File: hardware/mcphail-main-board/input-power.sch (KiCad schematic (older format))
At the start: 34 parts, among them J8 INPUT 6V-9V, J9 JST PH, U10 BUCK-BOOST 5V TPS63060, U11 MCP1703, U9 MCP73871

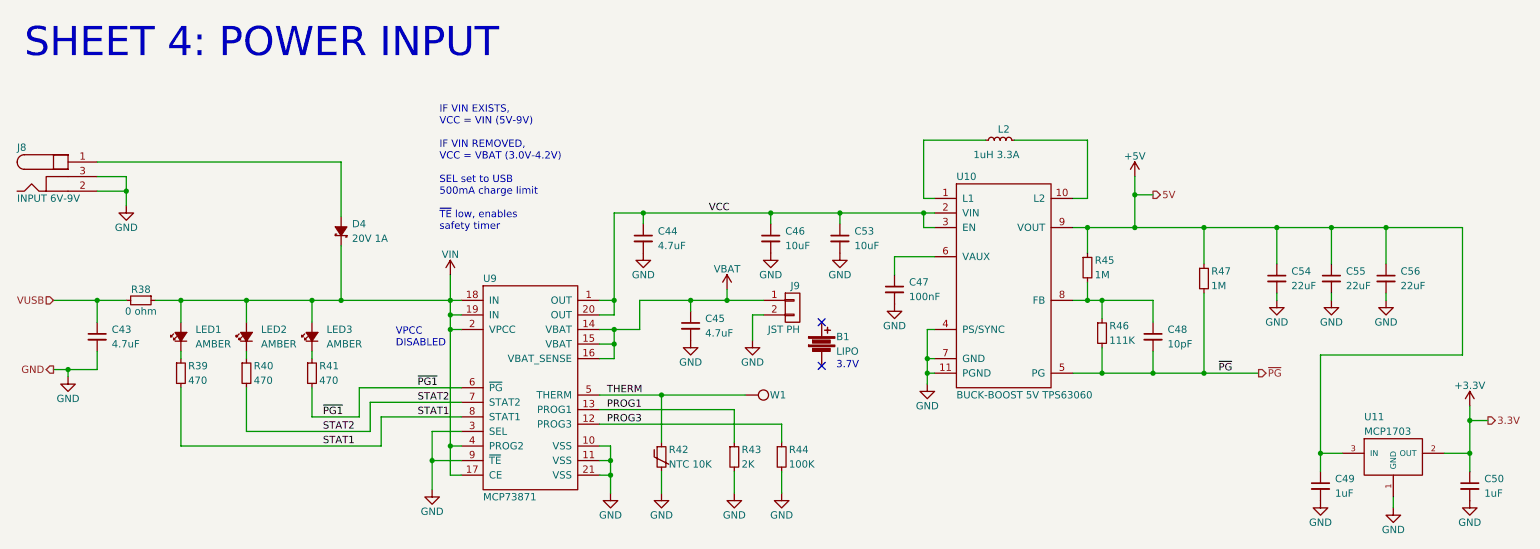
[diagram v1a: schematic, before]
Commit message: Commit.
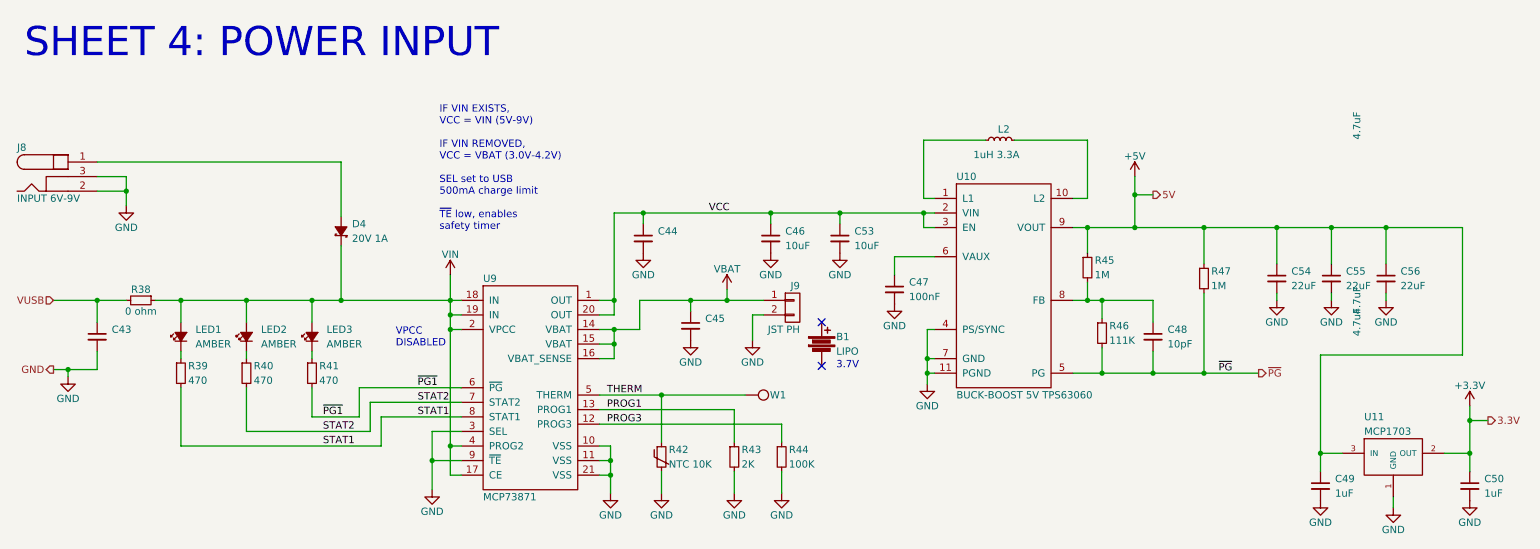
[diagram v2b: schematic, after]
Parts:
- C43, C44, C45: MF_Name Taiyo Yuden -> Samsung; MF_PN UMK316AB7475KL-T -> CL31B475KBHNNNE; S1_PN 587-2994-1-ND -> 1276-2789-1-ND
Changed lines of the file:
@@
 EESchema Schematic File Version 2
 LIBS:wickerlib
-LIBS:mcphail-main-board-cache
 EELAYER 25 0
 EELAYER END
@@
 P 4975 2325
 F 0 "C44" H 5075 2375 50  0000 L CNN
-F 1 "4.7uF" H 5075 2275 50  0000 L CNN
-F 2 "Wickerlib:RLC-1206-SMD" H 5600 1925 50  0001 C CIN
-F 3 "http://ds.yuden.co.jp/TYCOMPAS/ut/detail.do?productNo=UMK316AB7475KL-T&fileName=UMK316AB7475KL-T_SS&mode=specSheetDownload" H 5325 2100 50  0001 C CNN
-F 4 "CAP CER 4.7UF 50V X7R 1206" H 5650 2000 50  0001 C CIN "Description"
-F 5 "Taiyo Yuden" H 5175 1825 50  0001 C CIN "MF_Name"
-F 6 "UMK316AB7475KL-T" H 5850 1825 50  0001 C CIN "MF_PN"
-F 7 "Digikey" H 5075 1725 50  0001 C CIN "S1_Name"
-F 8 "587-2994-1-ND" H 5775 1725 50  0001 C CIN "S1_PN"
+F 1 "4.7uF" V 9875 3100 50  0000 C CNN
+F 2 "Wickerlib:RLC-1206-SMD" H 10375 2700 50  0001 C CIN
+F 3 "http://www.samsungsem.com/kr/support/product-search/mlcc/CL31B475KBHNNNE.jsp" H 10100 2875 50  0001 C CNN
+F 4 "CAP CER 4.7UF 50V X7R 1206" H 10425 2775 50  0001 C CIN "Description"
+F 5 "Samsung" H 9950 2600 50  0001 C CIN "MF_Name"
+F 6 "CL31B475KBHNNNE" H 10625 2600 50  0001 C CIN "MF_PN"
+F 7 "Digikey" H 9850 2500 50  0001 C CIN "S1_Name"
+F 8 "1276-2789-1-ND" H 10550 2500 50  0001 C CIN "S1_PN"
 	1    4975 2325
 	1    0    0    -1
@@
 P 5300 2925
 F 0 "C45" H 5400 2975 50  0000 L CNN
-F 1 "4.7uF" H 5400 2875 50  0000 L CNN
-F 2 "Wickerlib:RLC-1206-SMD" H 5925 2525 50  0001 C CIN
-F 3 "http://ds.yuden.co.jp/TYCOMPAS/ut/detail.do?productNo=UMK316AB7475KL-T&fileName=UMK316AB7475KL-T_SS&mode=specSheetDownload" H 5650 2700 50  0001 C CNN
-F 4 "CAP CER 4.7UF 50V X7R 1206" H 5975 2600 50  0001 C CIN "Description"
-F 5 "Taiyo Yuden" H 5500 2425 50  0001 C CIN "MF_Name"
-F 6 "UMK316AB7475KL-T" H 6175 2425 50  0001 C CIN "MF_PN"
-F 7 "Digikey" H 5400 2325 50  0001 C CIN "S1_Name"
-F 8 "587-2994-1-ND" H 6100 2325 50  0001 C CIN "S1_PN"
+F 1 "4.7uF" V 9875 3100 50  0000 C CNN
+F 2 "Wickerlib:RLC-1206-SMD" H 10375 2700 50  0001 C CIN
+F 3 "http://www.samsungsem.com/kr/support/product-search/mlcc/CL31B475KBHNNNE.jsp" H 10100 2875 50  0001 C CNN
+F 4 "CAP CER 4.7UF 50V X7R 1206" H 10425 2775 50  0001 C CIN "Description"
+F 5 "Samsung" H 9950 2600 50  0001 C CIN "MF_Name"
+F 6 "CL31B475KBHNNNE" H 10625 2600 50  0001 C CIN "MF_PN"
+F 7 "Digikey" H 9850 2500 50  0001 C CIN "S1_Name"
+F 8 "1276-2789-1-ND" H 10550 2500 50  0001 C CIN "S1_PN"
 	1    5300 2925
 	1    0    0    -1
@@
 P 1225 3000
 F 0 "C43" H 1325 3050 50  0000 L CNN
-F 1 "4.7uF" H 1325 2950 50  0000 L CNN
-F 2 "Wickerlib:RLC-1206-SMD" H 1850 2600 50  0001 C CIN
-F 3 "http://ds.yuden.co.jp/TYCOMPAS/ut/detail.do?productNo=UMK316AB7475KL-T&fileName=UMK316AB7475KL-T_SS&mode=specSheetDownload" H 1575 2775 50  0001 C CNN
-F 4 "CAP CER 4.7UF 50V X7R 1206" H 1900 2675 50  0001 C CIN "Description"
-F 5 "Taiyo Yuden" H 1425 2500 50  0001 C CIN "MF_Name"
-F 6 "UMK316AB7475KL-T" H 2100 2500 50  0001 C CIN "MF_PN"
-F 7 "Digikey" H 1325 2400 50  0001 C CIN "S1_Name"
-F 8 "587-2994-1-ND" H 2025 2400 50  0001 C CIN "S1_PN"
+F 1 "4.7uF" V 9875 3100 50  0000 C CNN
+F 2 "Wickerlib:RLC-1206-SMD" H 10375 2700 50  0001 C CIN
+F 3 "http://www.samsungsem.com/kr/support/product-search/mlcc/CL31B475KBHNNNE.jsp" H 10100 2875 50  0001 C CNN
+F 4 "CAP CER 4.7UF 50V X7R 1206" H 10425 2775 50  0001 C CIN "Description"
+F 5 "Samsung" H 9950 2600 50  0001 C CIN "MF_Name"
+F 6 "CL31B475KBHNNNE" H 10625 2600 50  0001 C CIN "MF_PN"
+F 7 "Digikey" H 9850 2500 50  0001 C CIN "S1_Name"
+F 8 "1276-2789-1-ND" H 10550 2500 50  0001 C CIN "S1_PN"
 	1    1225 3000
 	1    0    0    -1
